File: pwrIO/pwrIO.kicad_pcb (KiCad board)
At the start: 4 copper layers, 33.7 x 30.5 mm, 57 parts, among them IC3 TLV61225DC, J1 MOTOR1, J2 MOTOR2, J3 VCC_MOTOR, J4 MOTOR1, J5 MOTOR2, J6 MISC, J7 ENC1, J8 ENC2, U1 TB6612FNG, U2 TB6612FNG

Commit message: Updating pdf - adding blender export
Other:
- board text added: "PCB3D_BR_pwrIO"
- board text added: "PCB3D_TL_pwrIO"
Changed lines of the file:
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@@
 		)
+	)
+	(gr_text "PCB3D_BR_pwrIO"
+		(at 110.36 90.53 180)
+		(layer "Cmts.User")
+		(effects
+			(font
+				(size 1 1)
+				(thickness 0.2)
+				(bold yes)
+			)
+			(justify left bottom)
+		)
+	)
+	(gr_text "PCB3D_TL_pwrIO"
+		(at 76.71 60.03 0)
+		(layer "Cmts.User")
+		(effects
+			(font
+				(size 1 1)
+				(thickness 0.2)
+				(bold yes)
+			)
+			(justify left bottom)
+		)
+	)
+	(dimension
+		(type aligned)
+		(layer "Dwgs.User")
+		(pts
+			(xy 76.71 60.03) (xy 110.36 60.03)
+		)
+		(height -3.4)
+		(gr_text "33.6500 mm"
+			(at 93.535 55.48 0)
+			(layer "Dwgs.User")
+			(effects
+				(font
+					(size 1 1)
+					(thickness 0.15)
+				)
+			)
+		)
+		(format
+			(prefix "")
+			(suffix "")
+			(units 3)
+			(units_format 1)
+			(precision 4)
+		)
+		(style
+			(thickness 0.1)
+			(arrow_length 1.27)
+			(text_position_mode 0)
+			(extension_height 0.58642)
+			(extension_offset 0.5) keep_text_aligned)
+	)
+	(dimension
+		(type aligned)
+		(layer "Dwgs.User")
+		(pts
+			(xy 76.71 60.03) (xy 76.71 90.53)
+		)
+		(height 2.889999)
+		(gr_text "30.5000 mm"
+			(at 72.670001 75.28 90)
+			(layer "Dwgs.User")
+			(effects
+				(font
+					(size 1 1)
+					(thickness 0.15)
+				)
+			)
+		)
+		(format
+			(prefix "")
+			(suffix "")
+			(units 3)
+			(units_format 1)
+			(precision 4)
+		)
+		(style
+			(thickness 0.1)
+			(arrow_length 1.27)
+			(text_position_mode 0)
+			(extension_height 0.58642)
+			(extension_offset 0.5) keep_text_aligned)
 	)
 	(segment

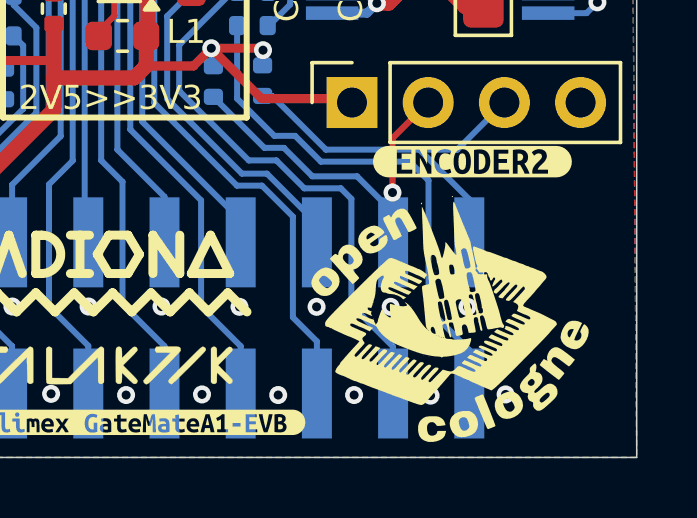
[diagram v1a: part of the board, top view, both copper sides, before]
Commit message: PCB update
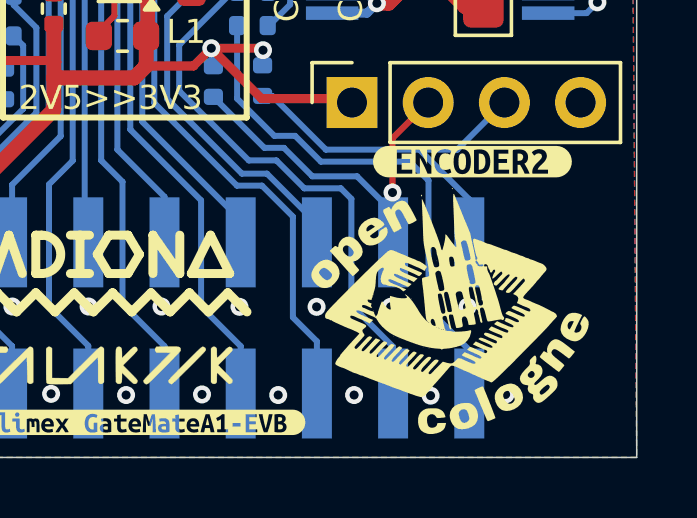
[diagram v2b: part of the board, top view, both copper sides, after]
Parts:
- moved H3 0.26 mm to (104.0, 85.7)
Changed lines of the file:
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@@
 		)
 		(property "Value" "100n"
-			(at 0 1.16 270)
+			(at 0 1.16 -90)
 			(layer "F.Fab")
 			(effects
@@
 		)
 		(fp_text user "${REFERENCE}"
-			(at 0 0 270)
+			(at 0 0 -90)
 			(layer "F.Fab")
 			(effects
@@
 		(tags "capacitor tantalum")
 		(property "Reference" "C8"
-			(at 3.072501 0.05 270)
+			(at 3.072501 0.05 -90)
 			(layer "F.SilkS")
 			(effects
@@
 		)
 		(property "Value" "10u"
-			(at 0 1.75 270)
+			(at 0 1.75 -90)
 			(layer "F.Fab")
 			(effects
@@
 		)
 		(fp_text user "${REFERENCE}"
-			(at 0 0 270)
+			(at 0 0 -90)
 			(layer "F.Fab")
 			(effects
@@
 	(footprint "Cologne:open_cologne"
 		(layer "F.Cu")
-		(at 104.02 85.94)
+		(at 104.02 85.675736)
 		(property "Reference" "H3"
 			(at 0 0 0)
@@
 		(tags "capacitor tantalum")
 		(property "Reference" "C9"
-			(at 3.082501 -0.02 270)
+			(at 3.082501 -0.02 -90)
 			(layer "F.SilkS")
 			(effects
@@
 		)
 		(property "Value" "10u"
-			(at 0 1.75 270)
+			(at 0 1.75 -90)
 			(layer "F.Fab")
 			(effects
@@
 		)
 		(fp_text user "${REFERENCE}"
-			(at 0 0 270)
+			(at 0 0 -90)
 			(layer "F.Fab")
 			(effects
@@
 		(tags "THT Terminal Block Phoenix MPT-0,5-2-2.54 pitch 2.54mm size 5.54x6.2mm^2 drill 1.1mm pad 2.2mm")
 		(property "Reference" "J4"
-			(at 1.319999 -1.93 360)
+			(at 1.319999 -1.93 0)
 			(layer "F.SilkS")
 			(effects
@@
 		)
 		(fp_text user "${REFERENCE}"
-			(at 1.27 1.999999 360)
+			(at 1.27 1.999999 0)
 			(layer "F.Fab")
 			(effects
@@
 		(tags "THT Terminal Block Phoenix MPT-0,5-2-2.54 pitch 2.54mm size 5.54x6.2mm^2 drill 1.1mm pad 2.2mm")
 		(property "Reference" "J5"
-			(at 1.409999 -2.05 360)
+			(at 1.409999 -2.05 0)
 			(layer "F.SilkS")
 			(effects
@@
 		)
 		(fp_text user "${REFERENCE}"
-			(at 1.27 1.999999 360)
+			(at 1.27 1.999999 0)
 			(layer "F.Fab")
 			(effects
@@
 		)
 		(property "Value" "10u"
-			(at 48.84 -12.709999 270)
+			(at 48.84 -12.709999 -90)
 			(layer "F.Fab")
 			(effects
@@
 		)
 		(fp_text user "${REFERENCE}"
-			(at -1.43 1.529999 270)
+			(at -1.43 1.529999 -90)
 			(layer "F.Fab")
 			(effects
